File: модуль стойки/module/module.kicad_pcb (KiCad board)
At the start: 2 copper layers, 33 x 16 mm, 7 parts

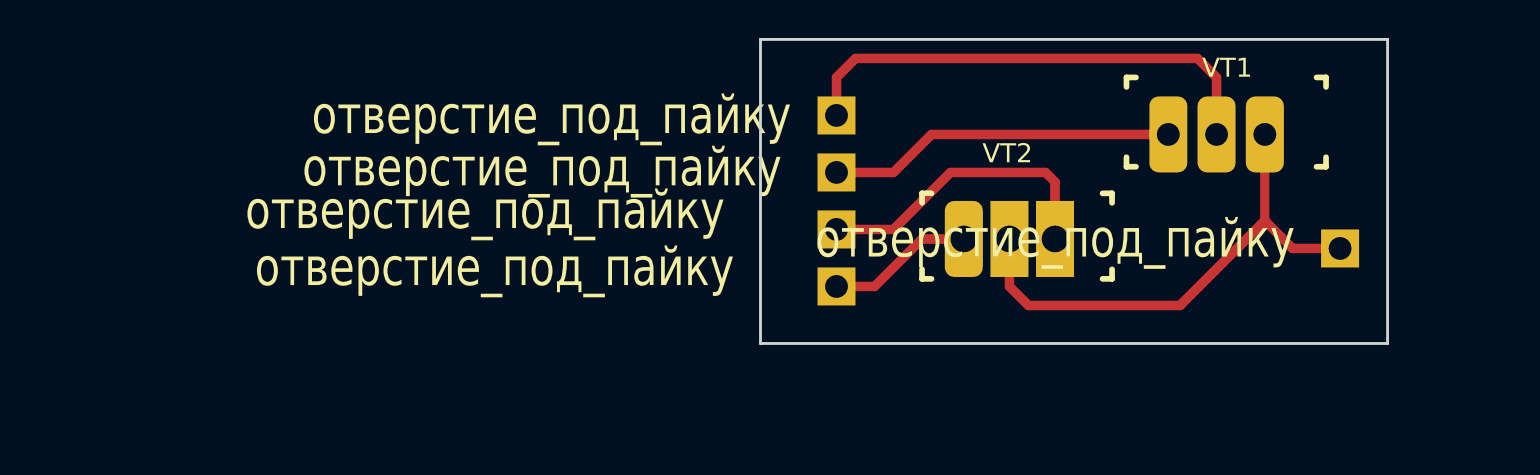
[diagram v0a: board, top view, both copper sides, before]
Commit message: модуль на стадии редактировании
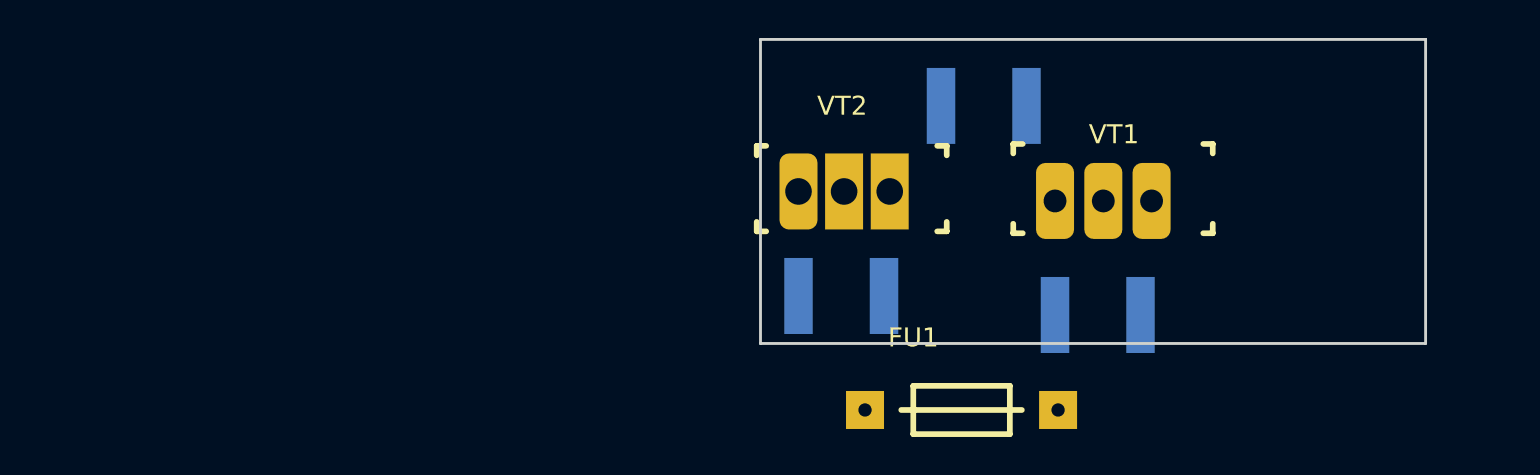
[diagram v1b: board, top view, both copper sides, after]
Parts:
- removed XS1, XS2, XS3, XS4, XS5: отверстие_под_пайку, MOTOR_ICO:Отверстие_под_пайку_D1.2
- added C1: Конденсатор_керамический, MOTOR_RLC:Конденсатор_SMD_1812, B.Cu at (151.0, 78.5)
- added C2: Конденсатор_керамический, MOTOR_RLC:Конденсатор_SMD_1812, B.Cu at (152.5, 89.5)
- added C3: Конденсатор_керамический, MOTOR_RLC:Конденсатор_SMD_1812, B.Cu at (139.0, 88.5)
- added FU1: Предохранитель, N_RLC:Предохранитель_R700, F.Cu at (142.5, 94.5)
- moved VT2 9.05 mm to (139.0, 83.0)
- moved VT1 6.91 mm to (152.5, 83.5)
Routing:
- net Net-(C2-Pad2): track 27.3 -> 0.00 mm
- net Net-(C3-Pad1): track 25.8 -> 0.00 mm
- net Net-(C2-Pad1): track 18.3 -> 0.00 mm
- net Net-(C1-Pad2): track 15.9 -> 0.00 mm
- net Net-(C1-Pad1): track 7.74 -> 0.00 mm
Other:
- board size 33 x 16 mm -> 35 x 16 mm
- net class Default: clearance 0.2 -> 0.4; trace_width 0.5 -> 0.4
- net class СИЛА added: clearance 0.4, trace_width 2.4, via_dia 0.8, via_drill 0.4
- rule trace_clearance: 0.2 -> 0.4
